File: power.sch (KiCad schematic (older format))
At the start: 16 parts, among them J10 USB_B_Micro, J9 Jack-DC, U12 MAX40203AUK, U13 MAX40203AUK

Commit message: Renamed to SMC-80
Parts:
- D11: symbol THS-80-rescue:LED-Device-max_breakout-rescue-sbc_z80-rescue -> SMC-80-rescue:LED-Device-max_breakout-rescue-sbc_z80-rescue
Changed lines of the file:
@@
 	2450 1600 3000 1600
 $Comp
-L THS-80-rescue:LED-Device-max_breakout-rescue-sbc_z80-rescue D?
+L SMC-80-rescue:LED-Device-max_breakout-rescue-sbc_z80-rescue D?
 U 1 1 5F826A18
 P 6200 1650

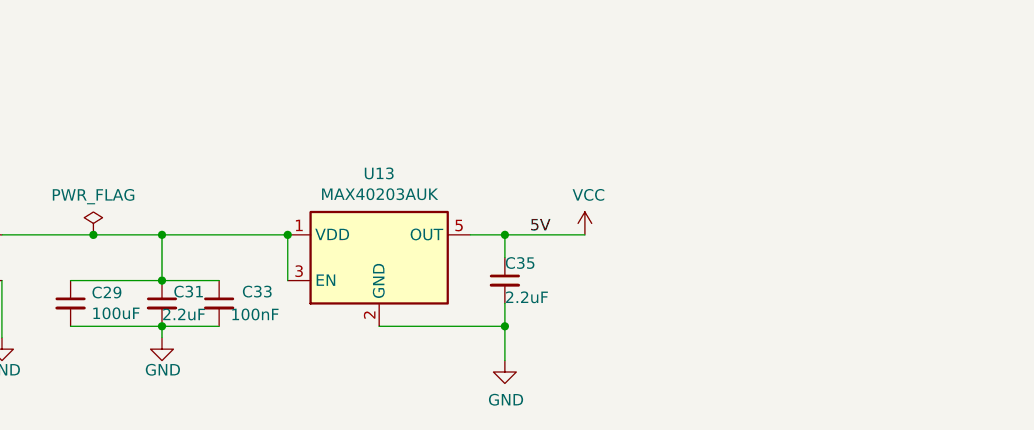
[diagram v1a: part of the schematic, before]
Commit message: trace routing
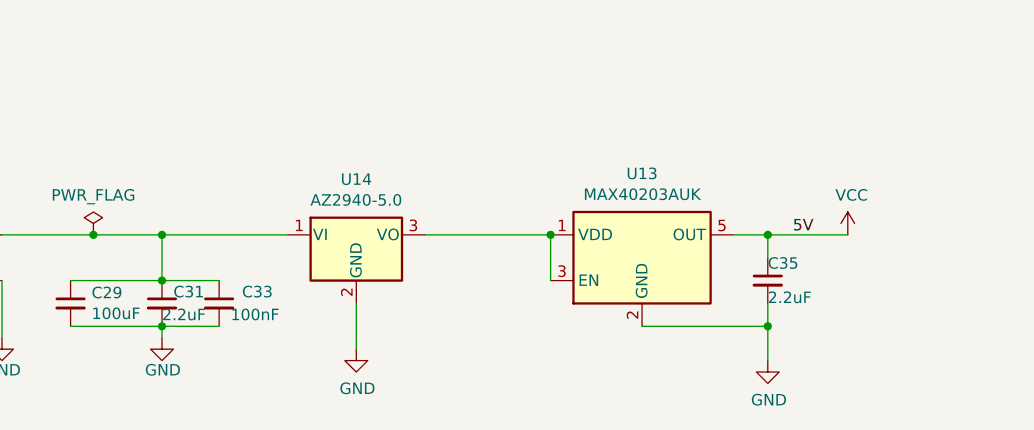
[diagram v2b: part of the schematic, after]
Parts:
- added U14: AZ2940-5.0, Package_TO_SOT_SMD:TO-252-2, symbol Regulator_Linear:AZ2940-5.0
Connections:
- net GND: now also U14.2 (GND)
- net at C29.1, C31.1, C33.1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: now also U14.1 (VI); no longer U13.1 (VDD), U13.3 (EN)
- new net: U13.1 (VDD), U13.3 (EN), U14.3 (VO)
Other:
- moved on the sheet: C35, U13
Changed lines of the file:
@@
 	1850 2200 1850 2600
 Wire Wire Line
-	3000 3700 3000 3900
-Wire Wire Line
-	3950 4000 3950 4100
-Connection ~ 3000 3700
+	4150 3700 4150 3900
+Wire Wire Line
+	5100 4000 5100 4100
+Connection ~ 4150 3700
 $Comp
 L Device:C_Small C?
 U 1 1 5F84975C
-P 3950 3900
+P 5100 3900
 AR Path="/5F84975C" Ref="C?"  Part="1"
 AR Path="/5F7E53CF/5F84975C" Ref="C35"  Part="1"
-F 0 "C35" H 3950 3975 50  0000 L CNN
-F 1 "2.2uF" H 3950 3825 50  0000 L CNN
-F 2 "Capacitor_SMD:C_0603_1608Metric_Pad1.05x0.95mm_HandSolder" H 3988 3750 50  0001 C CNN
-F 3 "https://www.mouser.com/datasheet/2/212/KEM_C1002_X7R_SMD-1102033.pdf" H 3950 3900 50  0001 C CNN
-F 4 "KEMET" H -2700 -2800 50  0001 C CNN "MFR"
-F 5 "C0805C105K4RACTU" H -2700 -2800 50  0001 C CNN "MPN"
-F 6 "Mouser" H -2700 -2800 50  0001 C CNN "SPR"
-F 7 "80-C0805C105K4R" H -2700 -2800 50  0001 C CNN "SPN"
-F 8 "https://www.mouser.com/ProductDetail/KEMET/C0805C105K8RAC7210?qs=sGAEpiMZZMs0AnBnWHyRQOf5HOpVaXbh6p7WVhSDTqQ%3D" H -2700 -2800 50  0001 C CNN "SPURL"
-	1    3950 3900
+F 0 "C35" H 5100 3975 50  0000 L CNN
+F 1 "2.2uF" H 5100 3825 50  0000 L CNN
+F 2 "Capacitor_SMD:C_0603_1608Metric_Pad1.05x0.95mm_HandSolder" H 5138 3750 50  0001 C CNN
+F 3 "https://www.mouser.com/datasheet/2/212/KEM_C1002_X7R_SMD-1102033.pdf" H 5100 3900 50  0001 C CNN
+F 4 "KEMET" H -1550 -2800 50  0001 C CNN "MFR"
+F 5 "C0805C105K4RACTU" H -1550 -2800 50  0001 C CNN "MPN"
+F 6 "Mouser" H -1550 -2800 50  0001 C CNN "SPR"
+F 7 "80-C0805C105K4R" H -1550 -2800 50  0001 C CNN "SPN"
+F 8 "https://www.mouser.com/ProductDetail/KEMET/C0805C105K8RAC7210?qs=sGAEpiMZZMs0AnBnWHyRQOf5HOpVaXbh6p7WVhSDTqQ%3D" H -1550 -2800 50  0001 C CNN "SPURL"
+	1    5100 3900
 	1    0    0    -1
 $EndComp
@@
 L Analog_Switch:MAX40200AUK U?
 U 1 1 5F849768
-P 3400 3800
+P 4550 3800
 AR Path="/5F849768" Ref="U?"  Part="1"
 AR Path="/5F7E53CF/5F849768" Ref="U13"  Part="1"
-F 0 "U13" H 3400 4167 50  0000 C CNN
-F 1 "MAX40203AUK" H 3400 4076 50  0000 C CNN
-F 2 "Package_TO_SOT_SMD:SOT-23-5_HandSoldering" H 3400 4300 50  0001 C CNN
-F 3 "https://datasheets.maximintegrated.com/en/ds/MAX40203.pdf" H 3400 4300 50  0001 C CNN
-F 4 "Maxim Integrated" H -250 -2300 50  0001 C CNN "MFR"
-F 5 "MAX40203AUK+T" H -250 -2300 50  0001 C CNN "MPN"
-F 6 "700-MAX40203AUK+T" H -250 -2300 50  0001 C CNN "Mouser PN"
-F 7 "700-MAX40200AUK+T" H -250 -2300 50  0001 C CNN "SPN"
-F 8 "Mouser" H -250 -2300 50  0001 C CNN "SPR"
-F 9 "https://www.mouser.com/ProductDetail/Maxim-Integrated/MAX40200AUK%2bT?qs=%2Fha2pyFadujABnCd8FHptN3rEsbd5utT%2FzHUaZs42SQ3v1htVXk3Hw%3D%3D" H -250 -2300 50  0001 C CNN "SPURL"
-	1    3400 3800
+F 0 "U13" H 4550 4167 50  0000 C CNN
+F 1 "MAX40203AUK" H 4550 4076 50  0000 C CNN
+F 2 "Package_TO_SOT_SMD:SOT-23-5_HandSoldering" H 4550 4300 50  0001 C CNN
+F 3 "https://datasheets.maximintegrated.com/en/ds/MAX40203.pdf" H 4550 4300 50  0001 C CNN
+F 4 "Maxim Integrated" H 900 -2300 50  0001 C CNN "MFR"
+F 5 "MAX40203AUK+T" H 900 -2300 50  0001 C CNN "MPN"
+F 6 "700-MAX40203AUK+T" H 900 -2300 50  0001 C CNN "Mouser PN"
+F 7 "700-MAX40200AUK+T" H 900 -2300 50  0001 C CNN "SPN"
+F 8 "Mouser" H 900 -2300 50  0001 C CNN "SPR"
+F 9 "https://www.mouser.com/ProductDetail/Maxim-Integrated/MAX40200AUK%2bT?qs=%2Fha2pyFadujABnCd8FHptN3rEsbd5utT%2FzHUaZs42SQ3v1htVXk3Hw%3D%3D" H 900 -2300 50  0001 C CNN "SPURL"
+	1    4550 3800
 	1    0    0    -1
 $EndComp
@@
 $EndComp
 Wire Wire Line
-	3950 3800 3950 3700
-Wire Wire Line
-	3950 4100 3950 4250
+	5100 3800 5100 3700
+Wire Wire Line
+	5100 4100 5100 4250
 $Comp
 L power:GND #PWR?
 U 1 1 5F849793
-P 3950 4250
+P 5100 4250
 AR Path="/5F849793" Ref="#PWR?"  Part="1"
 AR Path="/5CB63856/5F849793" Ref="#PWR?"  Part="1"
 AR Path="/5CB5AB00/5CB63856/5F849793" Ref="#PWR?"  Part="1"
 AR Path="/5F7E53CF/5F849793" Ref="#PWR088"  Part="1"
-F 0 "#PWR088" H 3950 4000 50  0001 C CNN
-F 1 "GND" H 3955 4077 50  0000 C CNN
-F 2 "" H 3950 4250 50  0001 C CNN
-F 3 "" H 3950 4250 50  0001 C CNN
-	1    3950 4250
-	1    0    0    -1
-$EndComp
-Wire Wire Line
-	3400 4100 3950 4100
-Wire Wire Line
-	3800 3700 3950 3700
-Connection ~ 3950 3700
-Connection ~ 3950 4100
+F 0 "#PWR088" H 5100 4000 50  0001 C CNN
+F 1 "GND" H 5105 4077 50  0000 C CNN
+F 2 "" H 5100 4250 50  0001 C CNN
+F 3 "" H 5100 4250 50  0001 C CNN
+	1    5100 4250
+	1    0    0    -1
+$EndComp
+Wire Wire Line
+	4550 4100 5100 4100
+Wire Wire Line
+	4950 3700 5100 3700
+Connection ~ 5100 3700
+Connection ~ 5100 4100
 $Comp
 L Device:C_Small C?
@@
 	2450 3700 2450 3900
 Wire Wire Line
-	2450 3700 3000 3700
+	3600 3700 4150 3700
 $Comp
 L power:PWR_FLAG #FLG?
@@
 L power:VCC #PWR?
 U 1 1 5F8497CA
-P 4300 3700
+P 5450 3700
 AR Path="/5F8497CA" Ref="#PWR?"  Part="1"
 AR Path="/5F7E53CF/5F8497CA" Ref="#PWR090"  Part="1"
-F 0 "#PWR090" H 4300 3550 50  0001 C CNN
-F 1 "VCC" H 4317 3873 50  0000 C CNN
-F 2 "" H 4300 3700 50  0001 C CNN
-F 3 "" H 4300 3700 50  0001 C CNN
-	1    4300 3700
-	1    0    0    -1
-$EndComp
-Wire Wire Line
-	3950 3700 4300 3700
-Text Label 4150 3700 2    50   ~ 0
+F 0 "#PWR090" H 5450 3550 50  0001 C CNN
+F 1 "VCC" H 5467 3873 50  0000 C CNN
+F 2 "" H 5450 3700 50  0001 C CNN
+F 3 "" H 5450 3700 50  0001 C CNN
+	1    5450 3700
+	1    0    0    -1
+$EndComp
+Wire Wire Line
+	5100 3700 5450 3700
+Text Label 5300 3700 2    50   ~ 0
 5V
 $Comp
@@
 Wire Wire Line
 	1750 3700 2150 3700
-Connection ~ 2450 3700
 Wire Wire Line
 	1750 3900 1750 4150
@@
 Wire Wire Line
 	2150 3700 2450 3700
+$Comp
+L Regulator_Linear:AZ2940-5.0 U14
+U 1 1 5E9CBE38
+P 3300 3700
+F 0 "U14" H 3300 3942 50  0000 C CNN
+F 1 "AZ2940-5.0" H 3300 3851 50  0000 C CNN
+F 2 "Package_TO_SOT_SMD:TO-252-2" H 3300 3950 50  0001 C CIN
+F 3 "https://www.diodes.com/assets/Datasheets/AZ1117.pdf" H 3300 3700 50  0001 C CNN
+	1    3300 3700
+	1    0    0    -1
+$EndComp
+Wire Wire Line
+	3000 3700 2450 3700
+Connection ~ 2450 3700
+Wire Wire Line
+	3300 4000 3300 4200
+$Comp
+L power:GND #PWR?
+U 1 1 5E9D0637
+P 3300 4200
+AR Path="/5E9D0637" Ref="#PWR?"  Part="1"
+AR Path="/5CB63856/5E9D0637" Ref="#PWR?"  Part="1"
+AR Path="/5CB5AB00/5CB63856/5E9D0637" Ref="#PWR?"  Part="1"
+AR Path="/5F7E53CF/5E9D0637" Ref="#PWR0101"  Part="1"
+F 0 "#PWR0101" H 3300 3950 50  0001 C CNN
+F 1 "GND" H 3305 4027 50  0000 C CNN
+F 2 "" H 3300 4200 50  0001 C CNN
+F 3 "" H 3300 4200 50  0001 C CNN
+	1    3300 4200
+	1    0    0    -1
+$EndComp
 $EndSCHEMATC

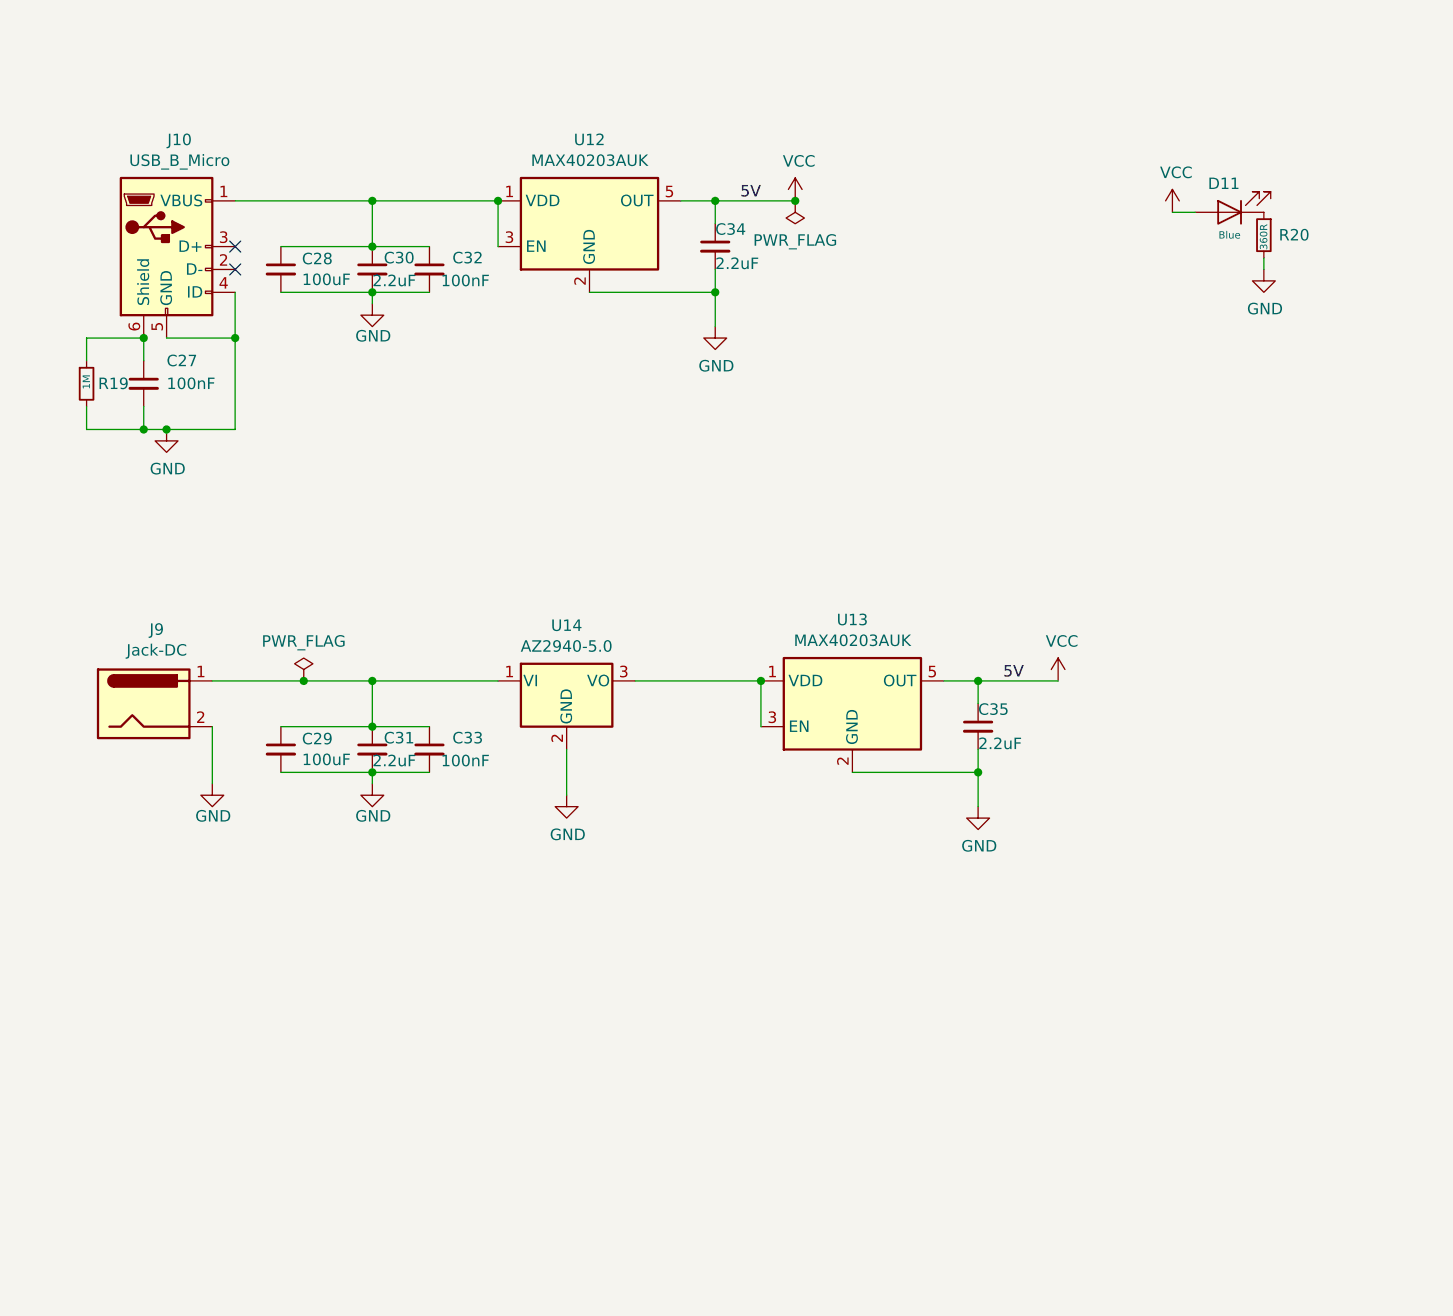
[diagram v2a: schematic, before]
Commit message: Routing finished
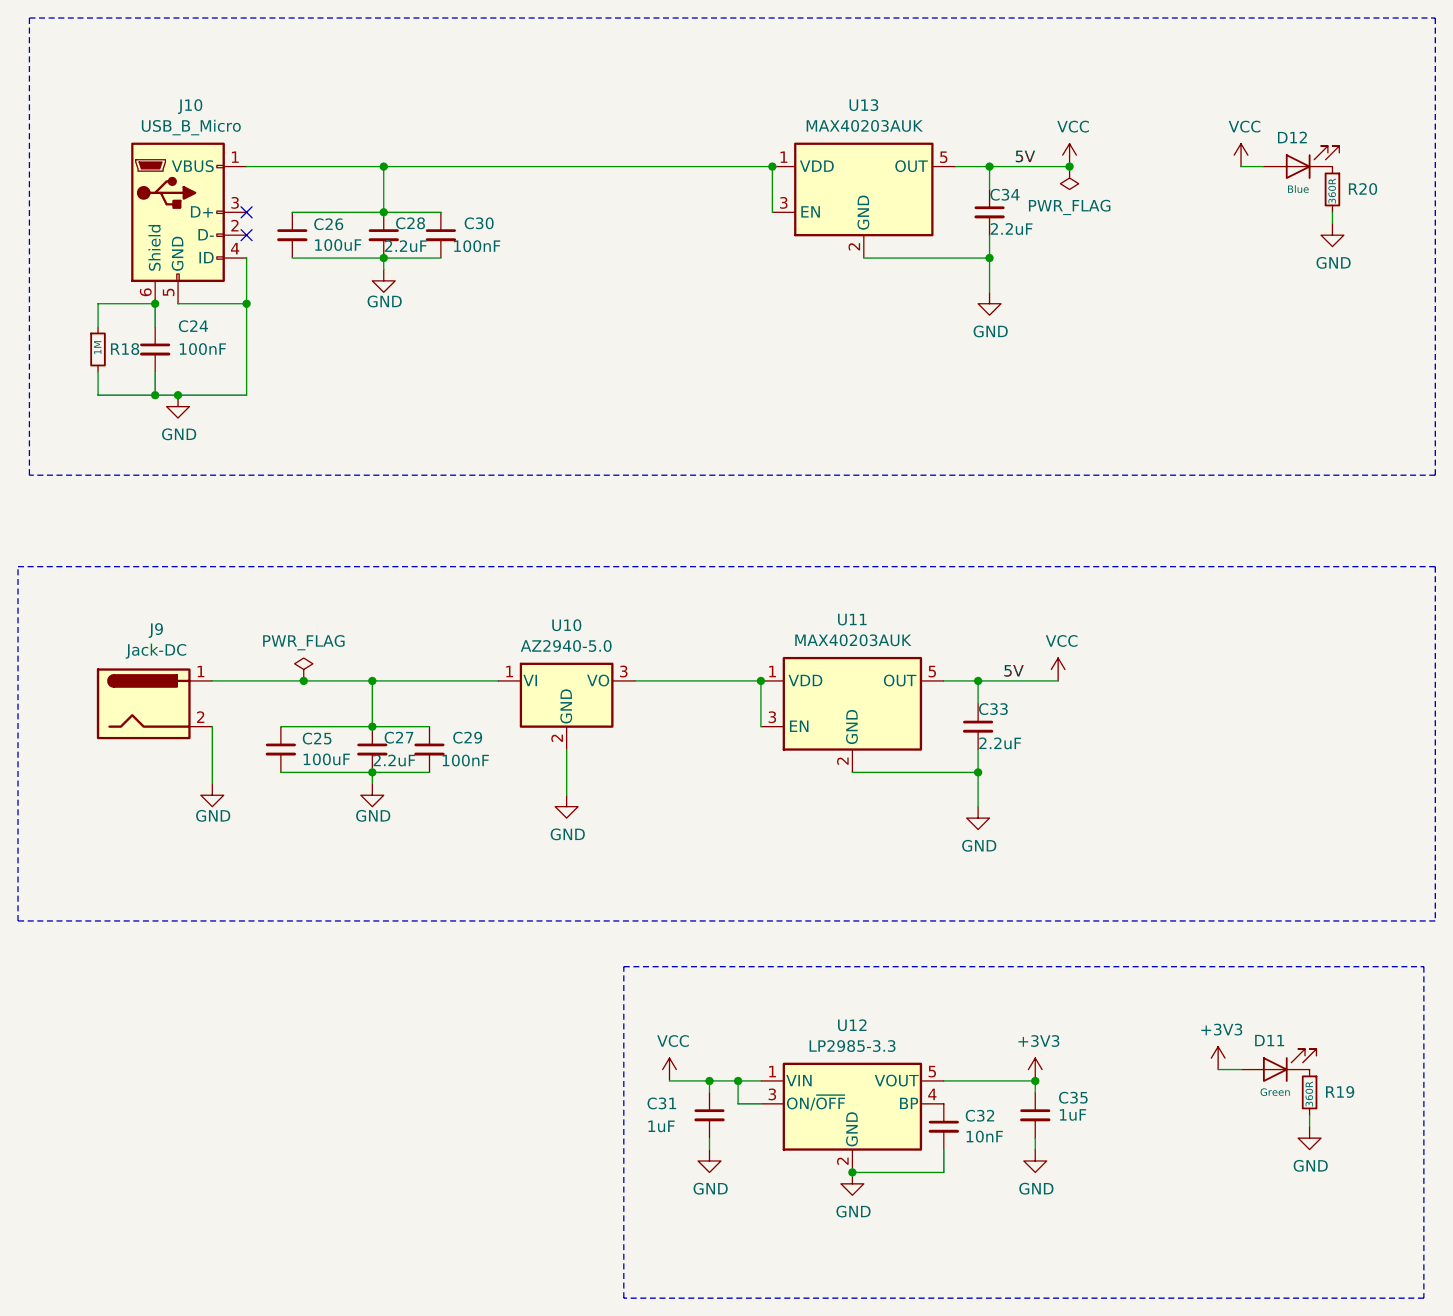
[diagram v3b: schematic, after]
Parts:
- added C31, C35: 1uF, Capacitor_SMD:C_0603_1608Metric_Pad1.05x0.95mm_HandSolder, symbol Device:C_Small
- added C32: 10nF, Capacitor_SMD:C_0603_1608Metric_Pad1.05x0.95mm_HandSolder, symbol Device:C_Small
- added D11: Green, LED_SMD:LED_0603_1608Metric_Pad1.05x0.95mm_HandSolder, symbol SMC-80-rescue:LED-Device-max_breakout-rescue-sbc_z80-rescue
- added R19: 360R, Resistor_SMD:R_0603_1608Metric_Pad1.05x0.95mm_HandSolder, symbol Device:R_Small
- added U12: LP2985-3.3, Package_TO_SOT_SMD:SOT-23-5, symbol Regulator_Linear:LP2985-3.3
- renumbered C27 to C24, C29 to C25, C28 to C26, C31 to C27, C30 to C28, C33 to C29, C32 to C30, C35 to C33, D11 to D12, R19 to R18, U14 to U10, U13 to U11, U12 to U13
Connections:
- net GND: now also C31.2, C32.2, C35.2, R19.2, U12.2 (GND)
- net VCC: now also C31.1, U12.1 (VIN), U12.3 (ON/~OFF~)
- new net: C32.1, U12.4 (BP)
- new net: D11.1 (K), R19.1
- new net +3V3: C35.1, D11.2 (A), U12.5 (VOUT)
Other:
- moved on the sheet: C24, C26, C28, C30, C34, D12, J10, R18, R20, U13
